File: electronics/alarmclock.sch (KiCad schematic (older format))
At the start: 24 parts, among them J1 SWD, J2 AudioJack2, J3 Conn_02x08_Top_Bottom, J4 SocketTop, J5 SocketBottom, J6 PinheaderTop, J7 PinheaderBottom, SW1 Reset, SW2 Rotary_Encoder_Switch, U1 STM32L011K4T6, Y1 24MHz

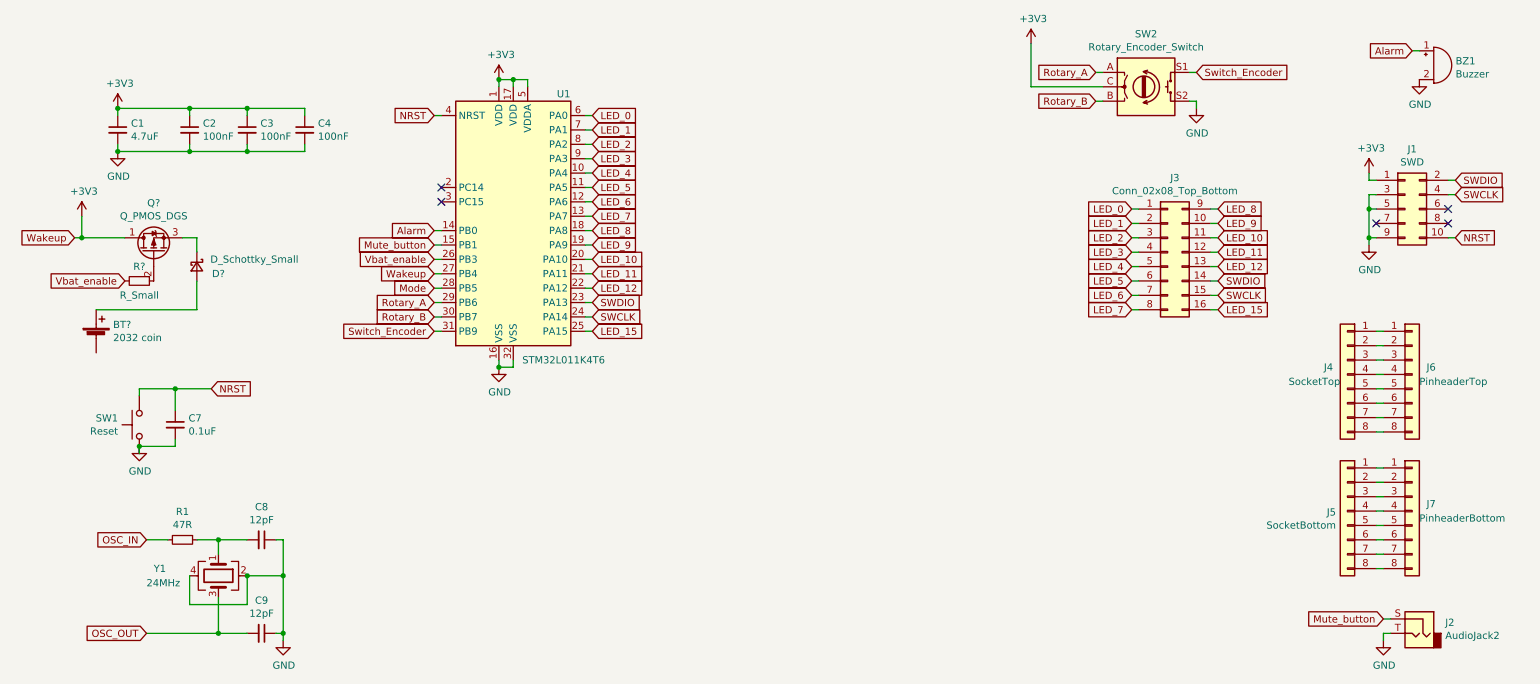
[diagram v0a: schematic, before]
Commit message: minor changes
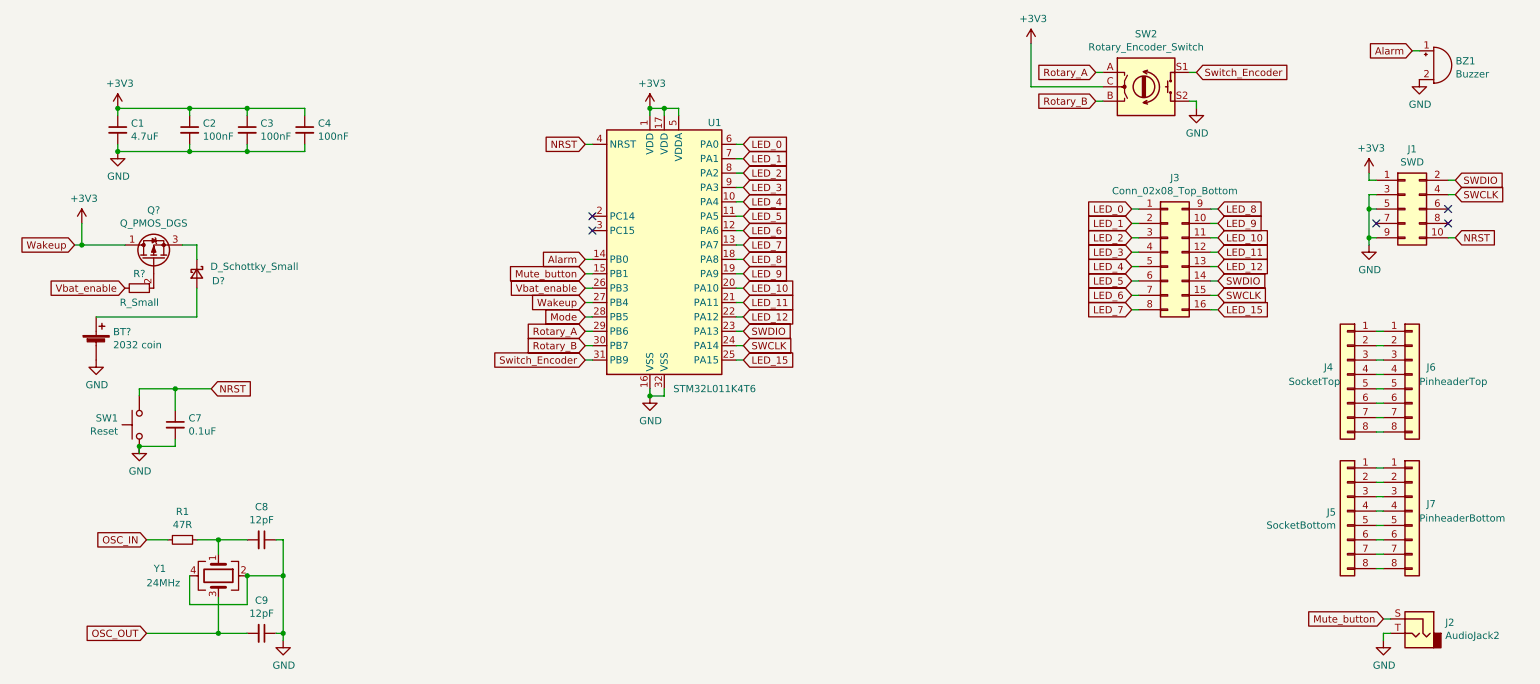
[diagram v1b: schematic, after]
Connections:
- net GND: now also BT?.2 (-)
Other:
- moved on the sheet: BT?, D?, Q?, R?, U1
